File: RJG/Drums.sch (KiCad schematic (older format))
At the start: 9 parts, among them U102 4520

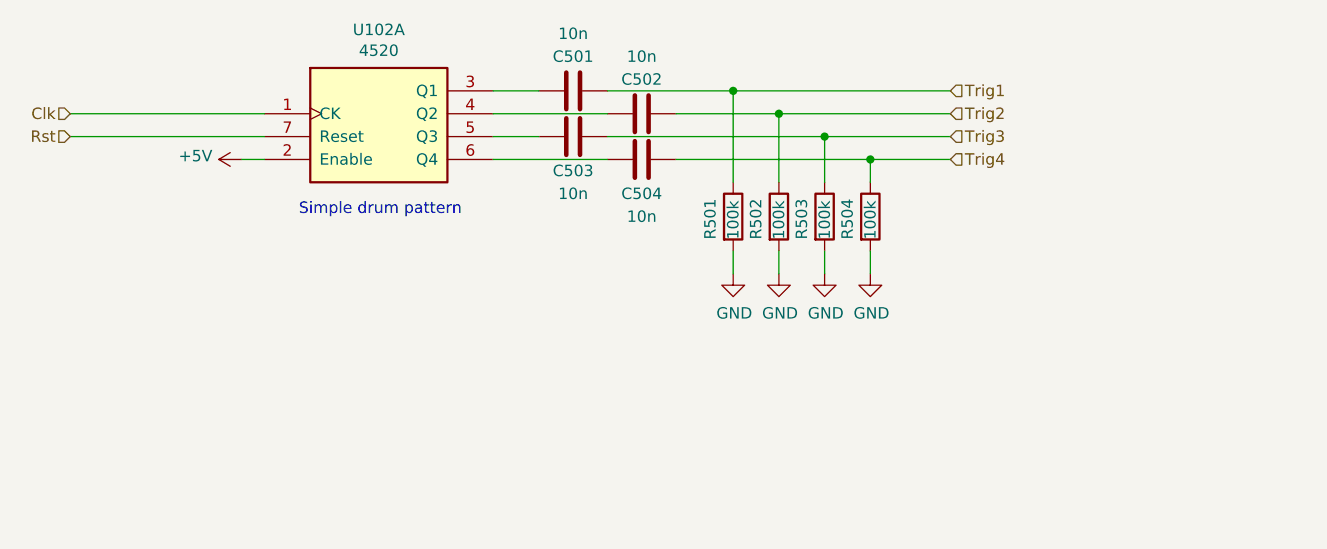
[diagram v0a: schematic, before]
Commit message: First layout fit
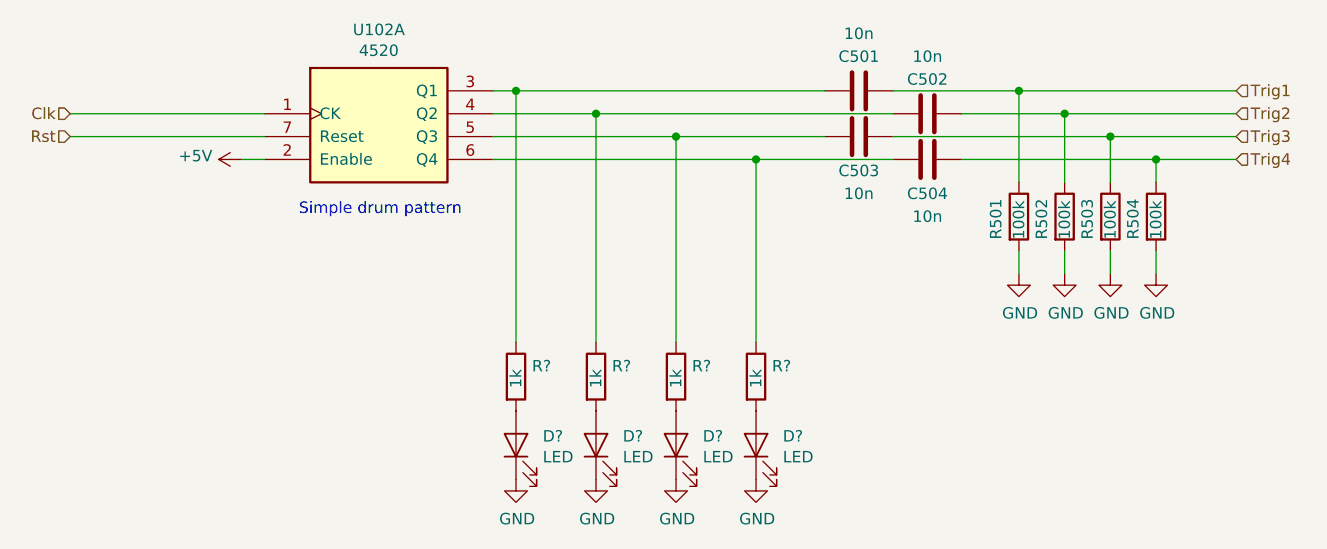
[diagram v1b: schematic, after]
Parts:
- added D? (x4): LED, LED_THT:LED_D3.0mm, symbol Device:LED
- added R? (x4): 1k, Resistor_THT:R_Axial_DIN0204_L3.6mm_D1.6mm_P7.62mm_Horizontal, symbol Device:R
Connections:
- net GND: now also D?.1 (K), D?.1 (K), D?.1 (K), D?.1 (K)
- net at C501.1, U102.3 (Q1): now also R?.1
- net at C502.1, U102.4 (Q2): now also R?.1
- net at C503.2, U102.5 (Q3): now also R?.1
- net at C504.2, U102.6 (Q4): now also R?.1
- new net: D?.2 (A), R?.2 (x4)
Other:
- moved on the sheet: C501, C502, C503, C504, R501, R502, R503, R504
